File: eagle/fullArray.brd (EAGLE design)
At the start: 43 x 72 mm, 119 parts

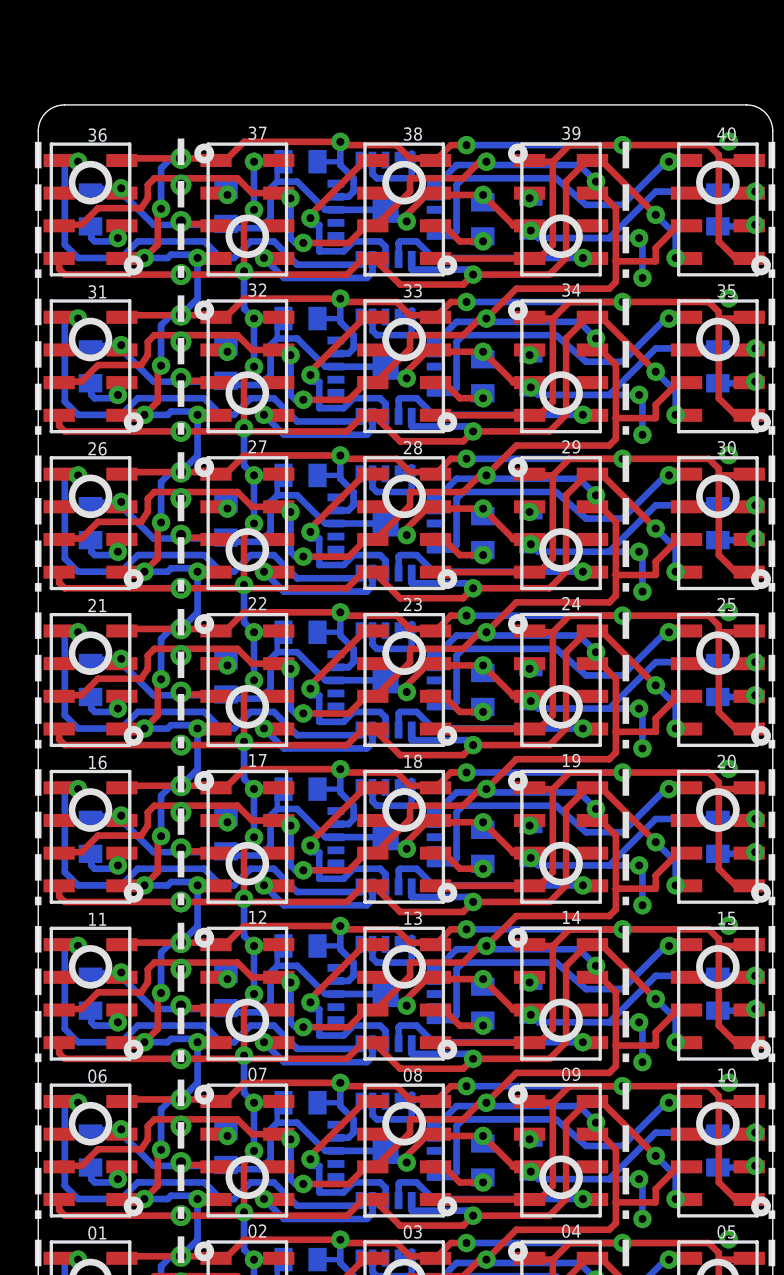
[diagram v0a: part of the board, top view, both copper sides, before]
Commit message: fixed addressing logic pin assignment, zero airwires, zero todos
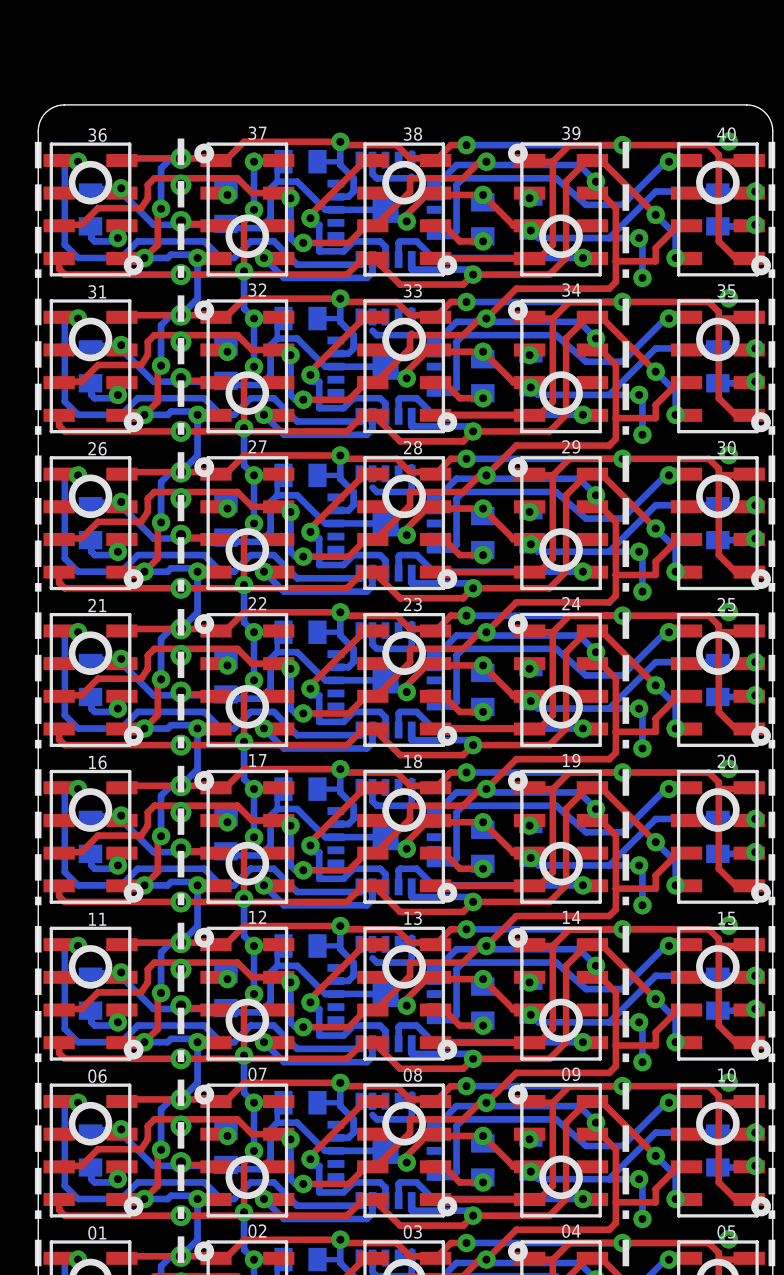
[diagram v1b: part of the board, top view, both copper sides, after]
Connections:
- removed net ADDR00: UC01.11, UC02.11, UC03.11, UC04.11, UC05.11, UC06.11, UC07.11, UC08.11
- new net ADDR1A: UC01.11
- new net ADDR2A: UC02.12
- new net ADDR3A: UC03.11
- new net ADDR3B: UC03.12
- new net ADDR4A: UC04.14
- new net ADDR5A: UC05.11
- new net ADDR5B: UC05.14
- new net ADDR6A: UC06.12
- new net ADDR6B: UC06.14
- new net ADDR7A: UC07.11
- new net ADDR7B: UC07.12
- new net ADDR7C: UC07.14
- new net ADDR8A: UC08.15
- net GND: now also UC02.11, UC04.11, UC06.11, UC08.11; no longer UC02.12, UC03.12, UC04.14, UC05.14, UC06.12, UC06.14, UC07.12, UC07.14, UC08.15
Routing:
- net GND: track 370.3 -> 364.2 mm
